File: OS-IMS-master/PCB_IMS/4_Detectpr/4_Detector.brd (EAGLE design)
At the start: 41.4 x 41.4 mm, 0 parts

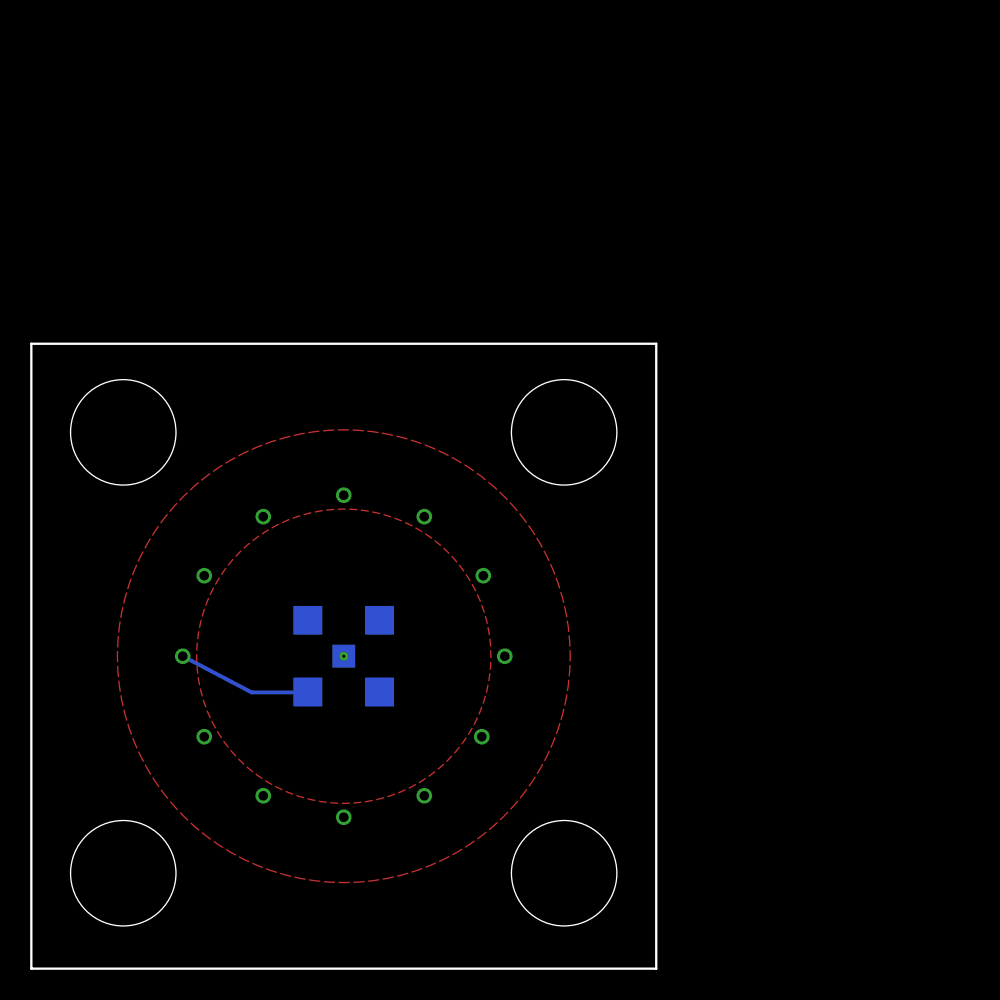
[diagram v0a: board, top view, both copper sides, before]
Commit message: chore: update boards on pcbway requests
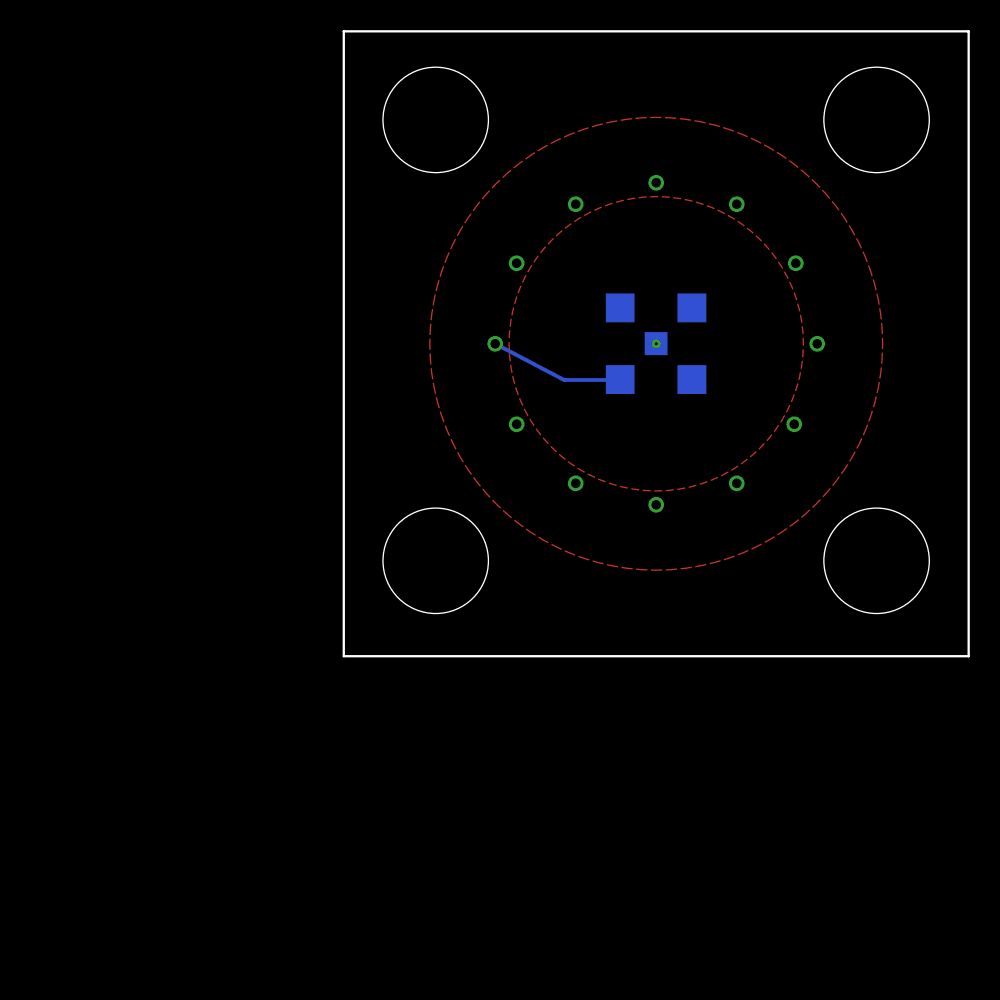
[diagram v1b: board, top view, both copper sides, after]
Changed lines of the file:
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@@
 <?xml version="1.0" encoding="utf-8"?>
 <!DOCTYPE eagle SYSTEM "eagle.dtd">
-<eagle version="8.3.0">
+<eagle version="9.2.2">
 <drawing>
 <settings>
@@
 <setting verticaltext="up"/>
 </settings>
-<grid distance="0.00393700787" unitdist="inch" unit="inch" style="lines" multiple="1" display="yes" altdistance="0.025" altunitdist="inch" altunit="inch"/>
+<grid distance="0.0999999999" unitdist="mm" unit="mm" style="lines" multiple="1" display="yes" altdistance="0.025" altunitdist="inch" altunit="inch"/>
 <layers>
 <layer number="1" name="Top" color="4" fill="1" visible="yes" active="yes"/>
@@
 <layer number="27" name="tValues" color="7" fill="1" visible="yes" active="yes"/>
 <layer number="28" name="bValues" color="7" fill="1" visible="yes" active="yes"/>
-<layer number="29" name="tStop" color="7" fill="3" visible="no" active="yes"/>
-<layer number="30" name="bStop" color="7" fill="6" visible="no" active="yes"/>
+<layer number="29" name="tStop" color="7" fill="3" visible="yes" active="yes"/>
+<layer number="30" name="bStop" color="7" fill="6" visible="yes" active="yes"/>
 <layer number="31" name="tCream" color="7" fill="4" visible="yes" active="yes"/>
 <layer number="32" name="bCream" color="7" fill="5" visible="yes" active="yes"/>
@@
 <board>
 <plain>
-<hole x="14.5996" y="14.83111875" drill="6.985"/>
-<hole x="-14.6104" y="14.83111875" drill="6.985"/>
-<hole x="-14.6104" y="-14.37888125" drill="6.985"/>
-<hole x="14.5996" y="-14.37888125" drill="6.985"/>
-<rectangle x1="-0.7677875" y1="-0.757640625" x2="0.7522125" y2="0.762359375" layer="16"/>
-<rectangle x1="-3.3377875" y1="-3.327640625" x2="-1.4277875" y2="-1.417640625" layer="16"/>
-<rectangle x1="-3.3377875" y1="1.422359375" x2="-1.4277875" y2="3.332359375" layer="16"/>
-<rectangle x1="1.4122125" y1="-3.327640625" x2="3.3222125" y2="-1.417640625" layer="16"/>
-<rectangle x1="1.4122125" y1="1.422359375" x2="3.3222125" y2="3.332359375" layer="16"/>
-<wire x1="-20.701" y1="-20.701" x2="-20.701" y2="20.701" width="0.1524" layer="20"/>
-<wire x1="-20.701" y1="20.701" x2="20.701" y2="20.701" width="0.1524" layer="20"/>
-<wire x1="20.701" y1="20.701" x2="20.701" y2="-20.701" width="0.1524" layer="20"/>
-<wire x1="-20.7" y1="-20.7" x2="20.7" y2="-20.7" width="0.1524" layer="20"/>
-<circle x="0" y="0" radius="14.008925" width="2.54" layer="29"/>
-<circle x="0" y="0" radius="11.5767" width="2.54" layer="29"/>
-<circle x="0.1" y="0" radius="9.3230875" width="2.54" layer="29"/>
-<circle x="0" y="-0.1" radius="7.2013875" width="2.54" layer="29"/>
-<circle x="0" y="0" radius="4.7927" width="2.54" layer="29"/>
-<circle x="0" y="0" radius="2.451528125" width="2.54" layer="29"/>
-<circle x="0" y="0" radius="0.1" width="2.54" layer="29"/>
-<rectangle x1="-3.4" y1="1.4" x2="-1.4" y2="3.4" layer="30"/>
-<rectangle x1="1.4" y1="1.4" x2="3.3" y2="3.3" layer="30"/>
-<rectangle x1="-0.8" y1="-0.8" x2="0.8" y2="0.8" layer="30"/>
-<rectangle x1="1.4" y1="-3.3" x2="3.3" y2="-1.4" layer="30"/>
-<rectangle x1="-3.3" y1="-3.3" x2="-1.4" y2="-1.4" layer="30"/>
+<hole x="35.2996" y="35.53111875" drill="6.985"/>
+<hole x="6.0896" y="35.53111875" drill="6.985"/>
+<hole x="6.0896" y="6.32111875" drill="6.985"/>
+<hole x="35.2996" y="6.32111875" drill="6.985"/>
+<rectangle x1="19.9322125" y1="19.942359375" x2="21.4522125" y2="21.462359375" layer="16"/>
+<rectangle x1="17.3622125" y1="17.372359375" x2="19.2722125" y2="19.282359375" layer="16"/>
+<rectangle x1="17.3622125" y1="22.122359375" x2="19.2722125" y2="24.032359375" layer="16"/>
+<rectangle x1="22.1122125" y1="17.372359375" x2="24.0222125" y2="19.282359375" layer="16"/>
+<rectangle x1="22.1122125" y1="22.122359375" x2="24.0222125" y2="24.032359375" layer="16"/>
+<wire x1="0" y1="0" x2="0" y2="41.4" width="0.1524" layer="20"/>
+<wire x1="0" y1="41.4" x2="41.4" y2="41.4" width="0.1524" layer="20"/>
+<wire x1="41.4" y1="41.4" x2="41.4" y2="0" width="0.1524" layer="20"/>
+<wire x1="0" y1="0" x2="41.4" y2="0" width="0.1524" layer="20"/>
+<circle x="20.7" y="20.7" radius="14.008925" width="2.54" layer="29"/>
+<circle x="20.7" y="20.7" radius="11.5767" width="2.54" layer="29"/>
+<circle x="20.8" y="20.7" radius="9.3230875" width="2.54" layer="29"/>
+<circle x="20.7" y="20.6" radius="7.2013875" width="2.54" layer="29"/>
+<circle x="20.7" y="20.7" radius="4.7927" width="2.54" layer="29"/>
+<circle x="20.7" y="20.7" radius="2.451528125" width="2.54" layer="29"/>
+<circle x="20.7" y="20.7" radius="0.1" width="2.54" layer="29"/>
+<rectangle x1="17.3" y1="22.1" x2="19.3" y2="24.1" layer="30"/>
+<rectangle x1="22.1" y1="22.1" x2="24" y2="24" layer="30"/>
+<rectangle x1="19.9" y1="19.9" x2="21.5" y2="21.5" layer="30"/>
+<rectangle x1="22.1" y1="17.4" x2="24" y2="19.3" layer="30"/>
+<rectangle x1="17.4" y1="17.4" x2="19.3" y2="19.3" layer="30"/>
 </plain>
 <attributes>
@@
 <param name="dpMaxLengthDifference" value="10mm"/>
 <param name="dpGapFactor" value="2.5"/>
-<param name="checkGrid" value="0"/>
 <param name="checkAngle" value="0"/>
 <param name="checkFont" value="1"/>
 <param name="checkRestrict" value="1"/>
+<param name="checkStop" value="0"/>
+<param name="checkValues" value="0"/>
+<param name="checkNames" value="1"/>
+<param name="checkWireStubs" value="1"/>
+<param name="checkPolygonWidth" value="0"/>
 <param name="useDiameter" value="13"/>
 <param name="maxErrors" value="50"/>
@@
 <signals>
 <signal name="S$4">
-<via x="-10.668" y="0" extent="1-16" drill="0.635"/>
-<wire x1="-10.668" y1="0" x2="-6.1" y2="-2.4" width="0.254" layer="16"/>
-<wire x1="-6.1" y1="-2.4" x2="-2.3" y2="-2.4" width="0.254" layer="16"/>
+<via x="10.032" y="20.7" extent="1-16" drill="0.635"/>
+<wire x1="10.032" y1="20.7" x2="14.6" y2="18.3" width="0.254" layer="16"/>
+<wire x1="14.6" y1="18.3" x2="18.4" y2="18.3" width="0.254" layer="16"/>
 <polygon width="0.1524" layer="1" rank="2">
-<vertex x="0" y="15" curve="90"/>
-<vertex x="-15" y="0" curve="90"/>
-<vertex x="0" y="-15" curve="90"/>
-<vertex x="15" y="0" curve="90"/>
+<vertex x="20.7" y="35.7" curve="90"/>
+<vertex x="5.7" y="20.7" curve="90"/>
+<vertex x="20.7" y="5.7" curve="90"/>
+<vertex x="35.7" y="20.7" curve="90"/>
 </polygon>
-<via x="9.2456" y="5.334" extent="1-16" drill="0.635"/>
-<via x="10.668" y="0" extent="1-16" drill="0.635"/>
-<via x="-9.2456" y="-5.334" extent="1-16" drill="0.635"/>
-<via x="0" y="-10.668" extent="1-16" drill="0.635"/>
-<via x="0" y="10.668" extent="1-16" drill="0.635"/>
-<via x="5.334" y="9.2456" extent="1-16" drill="0.635"/>
-<via x="9.144" y="-5.334" extent="1-16" drill="0.635"/>
-<via x="5.334" y="-9.2456" extent="1-16" drill="0.635"/>
-<via x="-5.334" y="-9.2456" extent="1-16" drill="0.635"/>
-<via x="-9.2456" y="5.334" extent="1-16" drill="0.635"/>
-<via x="-5.334" y="9.2456" extent="1-16" drill="0.635"/>
+<via x="29.9456" y="26.034" extent="1-16" drill="0.635"/>
+<via x="31.368" y="20.7" extent="1-16" drill="0.635"/>
+<via x="11.4544" y="15.366" extent="1-16" drill="0.635"/>
+<via x="20.7" y="10.032" extent="1-16" drill="0.635"/>
+<via x="20.7" y="31.368" extent="1-16" drill="0.635"/>
+<via x="26.034" y="29.9456" extent="1-16" drill="0.635"/>
+<via x="29.844" y="15.366" extent="1-16" drill="0.635"/>
+<via x="26.034" y="11.4544" extent="1-16" drill="0.635"/>
+<via x="15.366" y="11.4544" extent="1-16" drill="0.635"/>
+<via x="11.4544" y="26.034" extent="1-16" drill="0.635"/>
+<via x="15.366" y="29.9456" extent="1-16" drill="0.635"/>
 </signal>
 <signal name="S$3">
-<via x="0" y="0" extent="1-16" drill="0.2"/>
+<via x="20.7" y="20.7" extent="1-16" drill="0.2"/>
 <polygon width="0.1524" layer="1" orphans="yes">
-<vertex x="0" y="9.75" curve="90"/>
-<vertex x="-9.75" y="0" curve="90"/>
-<vertex x="0" y="-9.75" curve="90"/>
-<vertex x="9.75" y="0" curve="90"/>
+<vertex x="20.7" y="30.45" curve="90"/>
+<vertex x="10.95" y="20.7" curve="90"/>
+<vertex x="20.7" y="10.95" curve="90"/>
+<vertex x="30.45" y="20.7" curve="90"/>
 </polygon>
 </signal>
 </signals>
+<mfgpreviewcolors>
+<mfgpreviewcolor name="soldermaskcolor" color="0xC8008000"/>
+<mfgpreviewcolor name="silkscreencolor" color="0xFFFEFEFE"/>
+<mfgpreviewcolor name="backgroundcolor" color="0xFF282828"/>
+<mfgpreviewcolor name="coppercolor" color="0xFFFFBF00"/>
+<mfgpreviewcolor name="substratecolor" color="0xFF786E46"/>
+</mfgpreviewcolors>
 </board>
 </drawing>
